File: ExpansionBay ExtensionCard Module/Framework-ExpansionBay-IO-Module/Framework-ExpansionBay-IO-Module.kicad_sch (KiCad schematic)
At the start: 0 parts

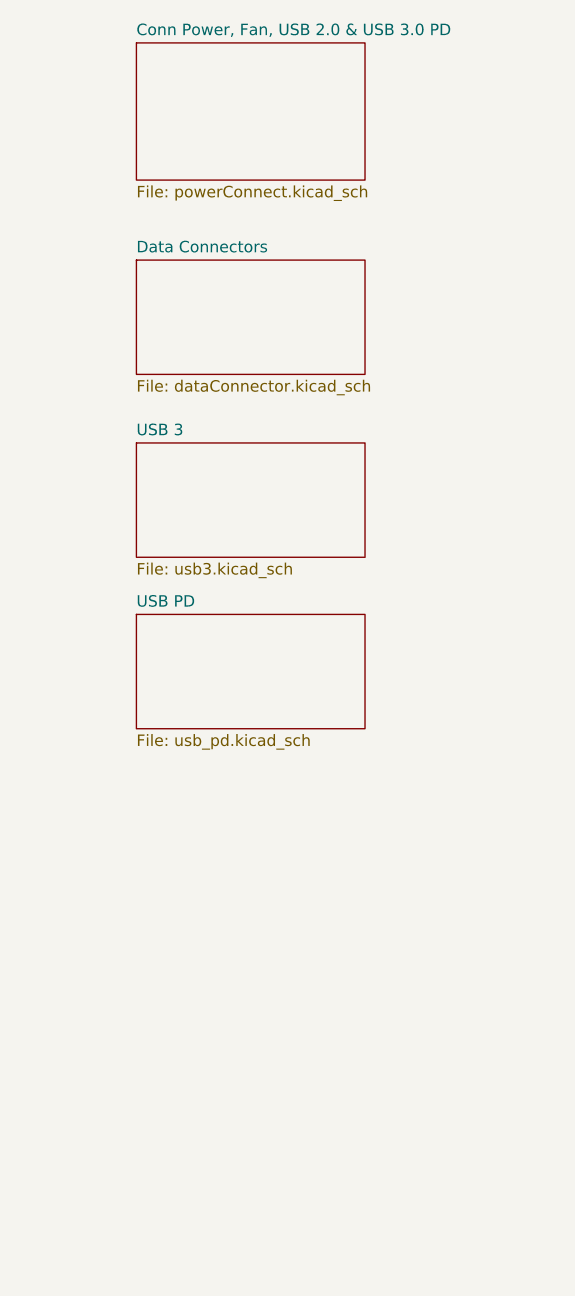
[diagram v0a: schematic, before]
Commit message: partial redesign
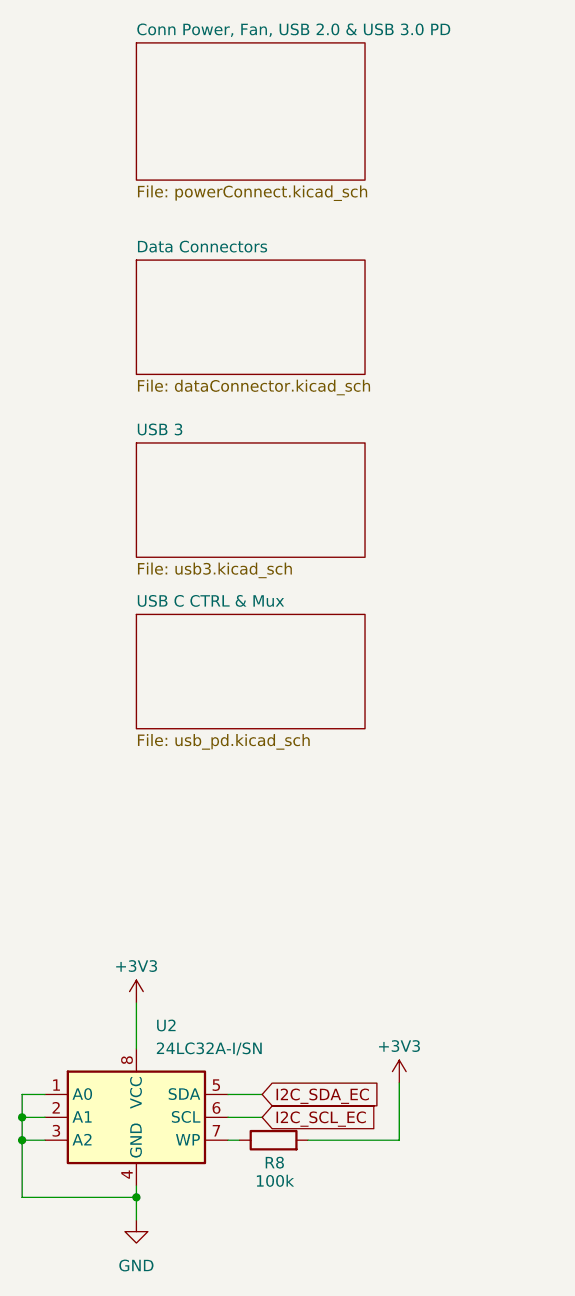
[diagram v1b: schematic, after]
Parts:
- added R8: 100k, Resistor_SMD:R_0805_2012Metric, symbol Device:R
- added U2: 24LC32A-I/SN, Package_SO:SOIC-8_3.9x4.9mm_P1.27mm, symbol Memory_EEPROM:24LC32
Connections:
- new net: R8.1, U2.7 (WP)
- new net +3V3: R8.2, U2.8 (VCC)
- new net GND: U2.1 (A0), U2.2 (A1), U2.3 (A2), U2.4 (GND)
- new net I2C_SCL_EC: U2.6 (SCL)
- new net I2C_SDA_EC: U2.5 (SDA)
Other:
- sheet USB PD renamed USB C CTRL & Mux
